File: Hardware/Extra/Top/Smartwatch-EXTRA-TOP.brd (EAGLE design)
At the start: 38 x 38 mm, 69 parts, among them SW6 SWITCH.MOM, SW7 SWITCH.MOM, U2 NRF52832_MODULE_MDBT42, U4 FT231XS, U5 PHOTOTRANSISTOR

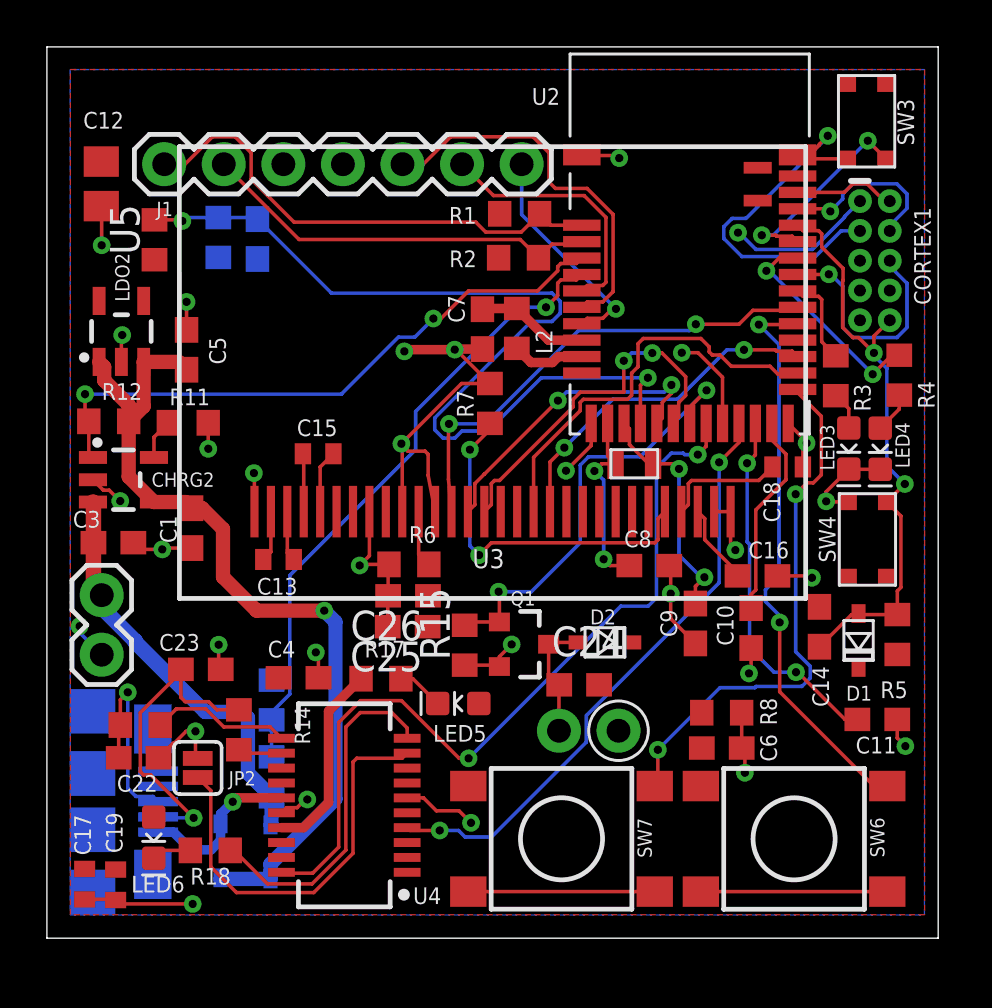
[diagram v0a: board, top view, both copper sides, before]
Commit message: Extra features updated
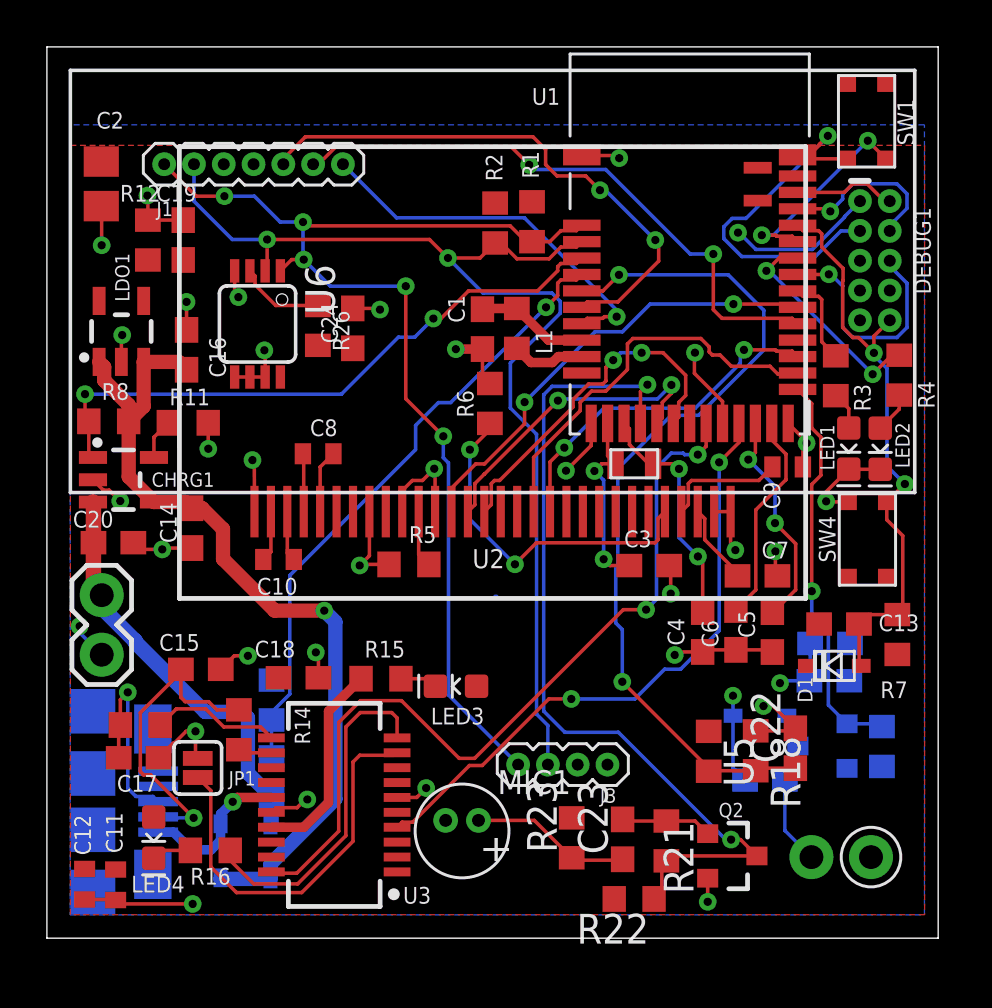
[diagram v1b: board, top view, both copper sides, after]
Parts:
- removed C25: 1u, LinnesLab-Passives:C0603
- removed C26: 100n, LinnesLab-Passives:C0603
- removed D4: (no value), LinnesLab-DiscreteSemi:USC
- removed LED5: RED, LinnesLab-LED:LED-0603
- removed LED6: YELLOW, LinnesLab-LED:LED-0603
- removed Q1: (no value), LinnesLab-DiscreteSemi:SOT23-3
- removed R17: 1k, LinnesLab-Passives:R0603
- removed SW6, SW7: SWITCH.MOM, LinnesLab-Switches:TACTILE_SWITCH_SMD_6.2MM_TALL
- removed U4: FT231XS, LinnesLab-DigitalIC:SSOP20_L
- added C2: 10u, LinnesLab-Passives:C0805
- added C27: 10p, LinnesLab-Passives:C0603
- added C28: 1u, LinnesLab-Passives:C0603
- added C29: 100n, LinnesLab-Passives:C0603
- added D3: (no value), LinnesLab-DiscreteSemi:USC
- added J3: (no value), LinnesLab-Connectors:1X04_1.27MM
- added LED1: RED, LinnesLab-LED:LED-0603
- added LED2: BLUE, LinnesLab-LED:LED-0603
- added MIC1: (no value), LinnesLab-Electromechanical:MICROPHONE_CMEJ-0415-42-P
- added Q2: (no value), LinnesLab-DiscreteSemi:SOT23-3@1
- added Q3: (no value), LinnesLab-DiscreteSemi:SOT23-3
- added R21: 100k, LinnesLab-Passives:R0603
- added R22, R23, R26: 10k, LinnesLab-Passives:R0603
- added R9: 27, LinnesLab-Passives:R0603
- added U1: NRF52832_MODULE_MDBT42, LinnesLab-Microcontrollers:BLE_MODULE_RAYTAC_MDBT42
- added U6: MCP9808-MSOP8, LinnesLab-Sensors:MSOP08
- C1: value 4.7u -> 1u
- C10, C11: value 300p -> 2.2uF; device LinnesLab-Passives:C0603 -> LinnesLab-Passives:C0402
- C12: value 10u -> 2.2uF; device LinnesLab-Passives:C0805 -> LinnesLab-Passives:C0402
- C13, C18: value 2.2uF -> 100n; device LinnesLab-Passives:C0402 -> LinnesLab-Passives:C0603
- C14: value 100n -> 4.7u
- C15, C17: value 2.2uF -> 47p; device LinnesLab-Passives:C0402 -> LinnesLab-Passives:C0603
- C16: value 10uF -> 1u
- C19: value 2.2uF -> 1u; device LinnesLab-Passives:C0402 -> LinnesLab-Passives:C0603
- C20: value 2.2u -> 4.7u
- C22: value 47p -> 2.2u
- C23: value 47p -> 100n
- C24: value 10p -> 100n
- C3: value 4.7u -> (none)
- C4: value 100n -> (none)
- C5, C6: value 1u -> 300p
- C7: value 1u -> 10uF
- C8, C9: value (none) -> 2.2uF; device LinnesLab-Passives:C0603 -> LinnesLab-Passives:C0402
- J1: device LinnesLab-Connectors:1X07 -> LinnesLab-Connectors:1X07_1.27MM
- LED4: value BLUE -> YELLOW
- R11: value (none) -> 4.7k
- R15: value 10k -> 1k
- R16: value 27 -> 1k
- R18: value 1k -> 10k
- R6: value 10k -> 390k
- R7: value 390k -> 10k
- U2: value NRF52832_MODULE_MDBT42 -> (none); device LinnesLab-Microcontrollers:BLE_MODULE_RAYTAC_MDBT42 -> LinnesLab-Displays:UG-2864HSWEG01_0.96IN_NO-WRAPAROUND
- U3: value (none) -> FT231XS; device LinnesLab-Displays:UG-2864HSWEG01_0.96IN_NO-WRAPAROUND -> LinnesLab-DigitalIC:SSOP20_L
- moved R19 35.7 mm to (35.6, 8.17)
- moved LED4 35.1 mm to (4.55, 4.29)
- moved C11 33.2 mm to (2.93, 2.28), turned to 90 degrees
- moved U5 32.2 mm to (28.2, 7.97), turned to 270 degrees
- moved C12 29.9 mm to (1.61, 2.30)
- moved R8 28.9 mm to (2.64, 22.0), turned to 0 degrees
- moved C22 28.0 mm to (31.9, 8.10), turned to 90 degrees
- moved C5 27.7 mm to (30.9, 13.1)
- moved C19 27.6 mm to (5.81, 29.8)
- moved C14 27.1 mm to (6.17, 17.5), turned to 90 degrees
- moved C16 26.2 mm to (5.95, 25.1), turned to 270 degrees
- moved C13 24.1 mm to (33.8, 13.4), turned to 0 degrees
- moved D5 23.7 mm to (30.4, 9.48), turned to 0 degrees
- moved R18 23.6 mm to (30.2, 7.99), turned to 270 degrees
- moved C3 22.9 mm to (25.7, 15.9), turned to 180 degrees
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- renumbered CHRG2 to CHRG1, CORTEX1 to DEBUG1, JP2 to JP1, L2 to L1, LDO2 to LDO1, SW3 to SW1, USB2 to USB1, XTAL2 to XTAL1
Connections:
- removed net A0/LIGHT: C20.1, R19.2, U2.15, U5.2
- removed net D11/SW1: SW7.A1, U2.25
- removed net D15/SW2: SW6.A1, U2.29
- removed net D29/LED.CTRL: J1.6, U2.6
- removed net D5/MOTOR: Q1.1, R15.2, U2.18
- removed net N$21: SW7.B1, SW7.B2
- removed net N$22: SW6.B1, SW6.B2
- new net A0/MICROPHONE: Q2.3, R21.2, R22.1, U1.15
- new net A5/LIGHT: C22.1, R18.2, U1.6, U5.2
- new net ALERT: R26.1, U6.3
- new net D11/MOTOR: Q3.1, R19.2, U1.25
- new net D15/LED.CTRL: J1.6, U1.29
- new net D5/CD1: U1.18
- new net N$19: C23.1, MIC1.+, R23.1
- new net N$20: C23.2, Q2.1, R21.1
- net !CTS: now also U3.9; no longer U4.9
- net !DTR: now also U3.1; no longer U4.1
- net 3.3V: now also C11.2, C18.2, C19.1, C2.2, C24.1, C27.2, C28.1, C29.1, D5.-, J3.2, LED3.A, LED4.A, R12.2, R22.2, R23.2, R26.2, R7.2, U1.11, U2.6, U2.9, U3.14, U3.3, U6.8; no longer C17.2, C19.2, C24.2, C25.1, C26.1, C4.2, C6.1, D2.-, LED5.A, LED6.A, R5.2, R8.2, U2.11, U3.6, U3.9, U4.14, U4.3
- net A4/BATT: now also U1.5; no longer U2.5
- net A6/TIA: now also U1.7; no longer U2.7
- net A7/PPG: now also U1.8; no longer U2.8
- net D16/CS.OLED: now also U1.30, U2.13; no longer U2.30, U3.13
- net D27/CHRG.STAT: now also R8.1, U1.4; no longer R12.1, U2.4
- net D3/RESET.OLED: now also U1.16, U2.14; no longer U2.16, U3.14
- net D4/DC.OLED: now also U1.17, U2.15; no longer U2.17, U3.15
- net D7/SD.CS: now also U1.20; no longer U2.20
- net DFU: now also U1.34; no longer U2.34
- net DTR: now also C13.1; no longer C14.1
- net FRST: now also U1.38; no longer U2.38
- net FT3V3: now also U3.13; no longer U4.13
- net GND: now also C1.2, C11.1, C14.1, C15.1, C17.2, C19.2, C2.1, C24.2, C28.2, C29.2, C3.1, C4.2, C5.2, C7.1, C9.1, J3.1, LED1.C, LED2.C, MIC1.-, Q2.2, Q3.2, R12.1, R18.1, R5.1, R6.2, U1.1, U1.12, U1.24, U1.39, U2.10, U2.29, U2.30, U2.8, U3.16, U3.6, U6.4, U6.5, U6.6, U6.7; no longer C1.1, C10.2, C11.2, C17.1, C19.1, C23.1, C25.2, C26.2, C3.2, C4.1, C5.1, C7.2, C8.1, C9.2, LED3.C, LED4.C, Q1.2, R15.1, R6.1, R7.2, R8.1, U2.24, U2.39, U3.1, U3.10, U3.12, U3.29, U3.30, U3.8, U4.16, U4.6
- net LED1: now also U1.31; no longer U2.31
- net LED2: now also U1.33; no longer U2.33
- net MISO: now also U1.28; no longer U2.28
- net MOSI: now also U1.27, U2.19; no longer U2.27, U3.19
- net N$1: now also R5.2, U2.11; no longer R6.2, U3.11
- net N$10: now also LED2.A; no longer LED4.A
- net N$11: now also U1.10; no longer U2.10
- net N$12: now also C1.1, U1.9; no longer C7.1, U2.9
- net N$13: now also C7.2, U2.28; no longer C16.2, U3.28
- net N$15: now also C9.2, U2.27; no longer C18.2, U3.27
- net N$18: now also C27.1, D5.+, Q3.3; no longer C24.1, D2.+, Q1.3
- net N$2: now also R6.1, U2.26; no longer R7.1, U3.26
- net N$25: now also R9.2, U3.12; no longer R10.2, U4.12
- net N$26: now also R10.2, U3.11; no longer R16.2, U4.11
- net N$27: now also LED3.C, R15.2; no longer LED5.C, R17.2
- net N$28: now also LED4.C, R16.2; no longer LED6.C, R18.2
- net N$3: now also C10.2, U2.2; no longer C13.2, U3.2
- net N$4: now also C3.2, U1.13; no longer C8.2, U2.13
- net N$5: now also C10.1, U2.3; no longer C13.1, U3.3
- net N$6: now also C4.1, U1.14; no longer C9.1, U2.14
- net N$7: now also C8.2, U2.4; no longer C15.2, U3.4
- net N$8: now also C8.1, U2.5; no longer C15.1, U3.5
- net N$9: now also LED1.A; no longer LED3.A
- net P0.09/NFC1: now also C5.1, U1.22; no longer C11.1, U2.22
- net P0.10/NFC2: now also C6.1, U1.23; no longer C10.1, U2.23
- net RESET: now also C13.2, R7.1, U1.35; no longer C14.2, R5.1, U2.35
- net RXD: now also U1.21, U3.4; no longer U2.21, U4.4
- net RXLED: now also R15.1, U3.17; no longer R17.1, U4.17
- net SCK: now also U1.26, U2.18; no longer U2.26, U3.18
- net SCL: now also J3.3, U1.3, U6.2; no longer U2.3
- net SDA: now also J3.4, U1.2, U6.1; no longer U2.2
- net SWCLK: now also U1.36; no longer U2.36
- net SWDIO: now also U1.37; no longer U2.37
- net SWO: now also U1.32; no longer U2.32
- net TXD: now also U1.19, U3.20; no longer U2.19, U4.20
- net TXLED: now also R16.1, U3.10; no longer R18.1, U4.10
- net USB+: now also C17.1, R10.1; no longer C22.1, R16.1
- net USB-: now also C15.2, R9.1; no longer C23.2, R10.1
- net VIN: now also C14.2, C16.2, D2.-, D3.-, R8.2; no longer C1.2, C5.2, D4.-, D5.-, R12.2
- net VLIPO: now also C20.1, D2.+; no longer C3.1, D4.+
- net V_USB: now also D3.+, U3.15; no longer D5.+, U4.15
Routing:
- net A0/LIGHT: track 39.4 -> 0.00 mm, vias 2 -> 0
- net A0/MICROPHONE: track 0.00 -> 37.3 mm, vias 0 -> 2
- net A5/LIGHT: track 0.00 -> 37.2 mm, vias 0 -> 2
- net SCL: track 17.2 -> 48.2 mm, vias 0 -> 2
- net SDA: track 21.2 -> 49.5 mm, vias 0 -> 5
- net D15/LED.CTRL: track 0.00 -> 25.5 mm, vias 0 -> 2
- net D15/SW2: track 24.4 -> 0.00 mm, vias 2 -> 0
- net D11/SW1: track 23.0 -> 0.00 mm, vias 2 -> 0
- net D5/MOTOR: track 18.9 -> 0.00 mm, vias 2 -> 0
- net D11/MOTOR: track 0.00 -> 17.0 mm, vias 0 -> 1
- net D29/LED.CTRL: track 11.0 -> 0.00 mm
- net N$22: track 7.95 -> 0.00 mm
- net N$21: track 7.95 -> 0.00 mm
- net A6/TIA: track 16.5 -> 23.7 mm, vias 0 -> 2
- net GND: track 93.4 -> 86.2 mm, vias 30 -> 32
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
